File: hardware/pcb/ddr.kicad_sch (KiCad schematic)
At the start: 6 parts, among them U8 MT41K256M16TW

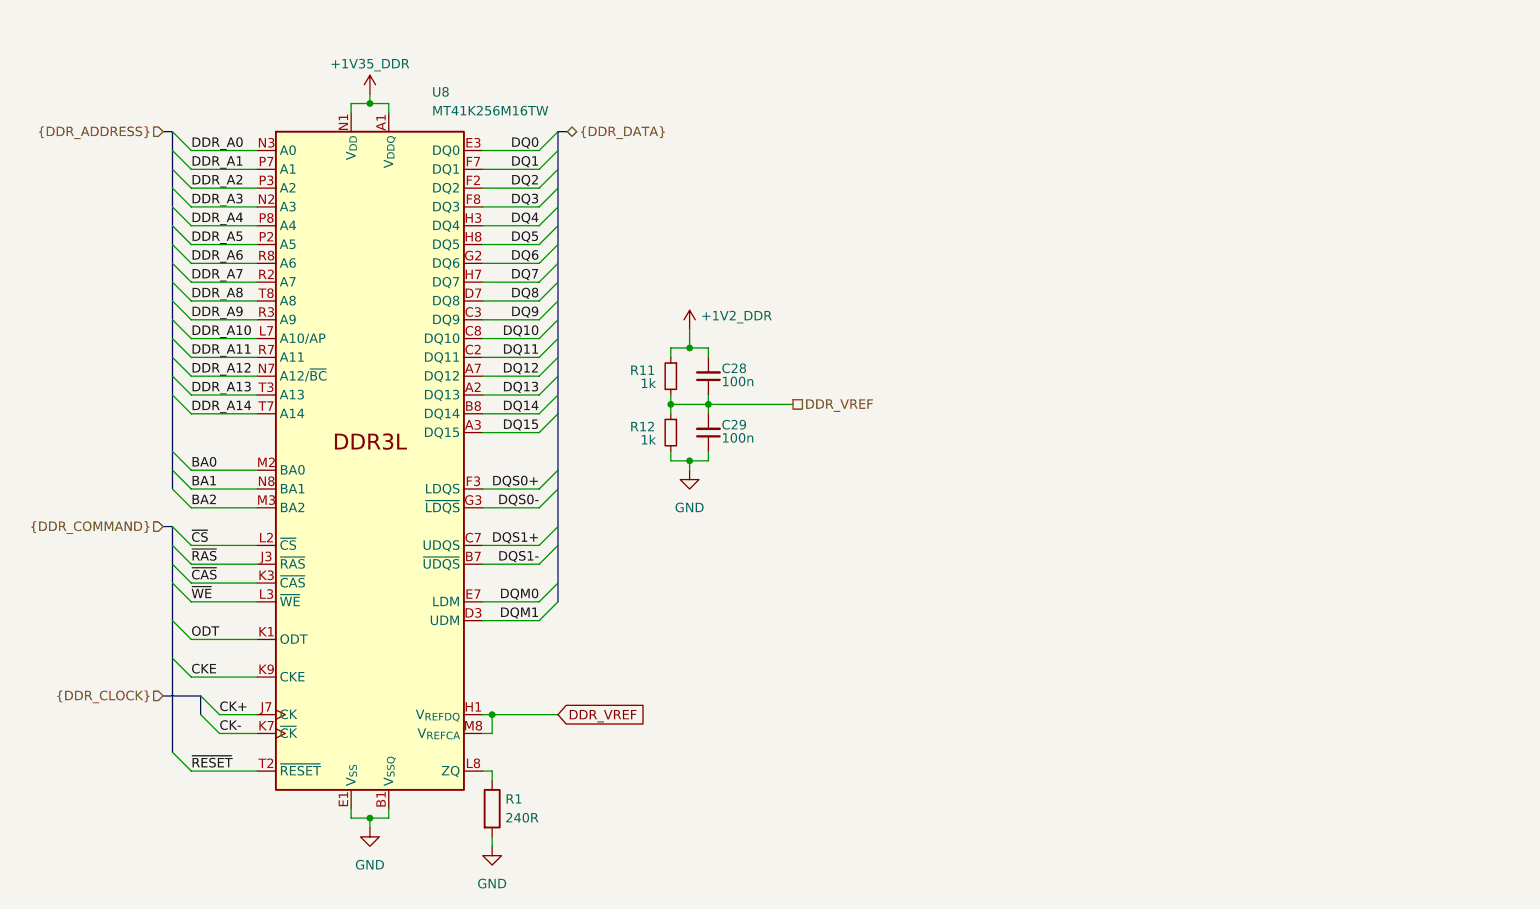
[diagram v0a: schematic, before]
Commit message: looking over stuff, added caps
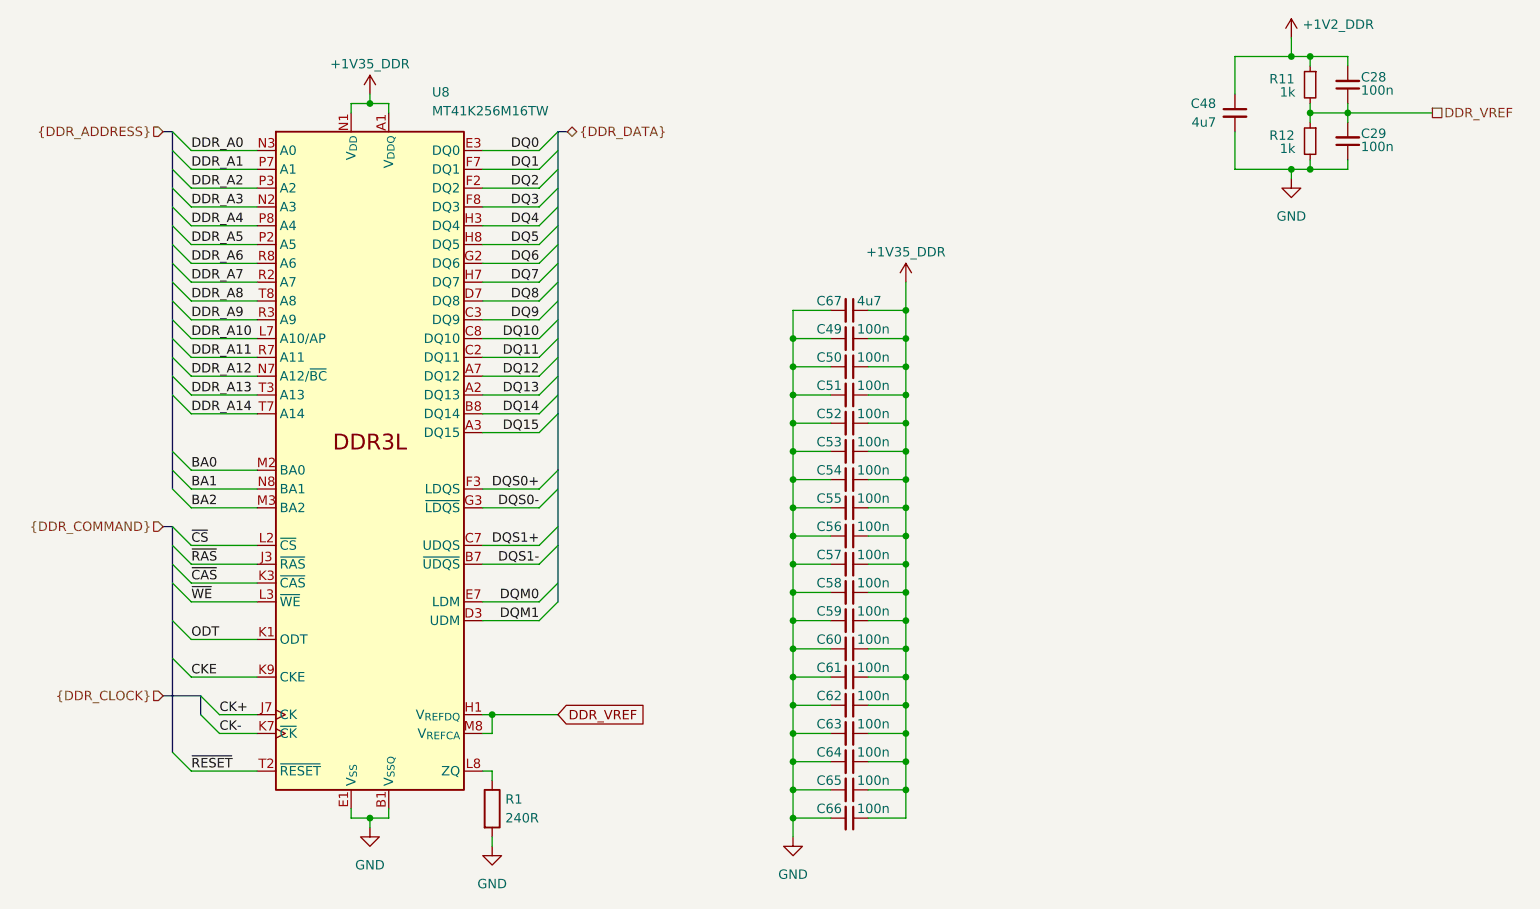
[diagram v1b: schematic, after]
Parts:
- added C48, C67: 4u7, Capacitor_SMD:C_0402_1005Metric, symbol Device:C_Small
- added C49, C50, C51, C52, C53, C54, C55, C56, C57, C58, C59, C60, C61, C62, C63, C64, C65, C66: 100n, Capacitor_SMD:C_0402_1005Metric, symbol Device:C_Small
- C28, C29: footprint (none) -> Capacitor_SMD:C_0402_1005Metric
- R1, R11, R12: footprint (none) -> Resistor_SMD:R_0402_1005Metric
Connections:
- net +1V2_DDR: now also C48.1
- net +1V35_DDR: now also C49.1, C50.1, C51.1, C52.1, C53.1, C54.1, C55.1, C56.1, C57.1, C58.1, C59.1, C60.1, C61.1, C62.1, C63.1, C64.1, C65.1, C66.1, C67.1
- net GND: now also C48.2, C49.2, C50.2, C51.2, C52.2, C53.2, C54.2, C55.2, C56.2, C57.2, C58.2, C59.2, C60.2, C61.2, C62.2, C63.2, C64.2, C65.2, C66.2, C67.2
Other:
- moved on the sheet: C28, C29, R11, R12
